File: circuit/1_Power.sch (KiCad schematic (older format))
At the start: 4 parts

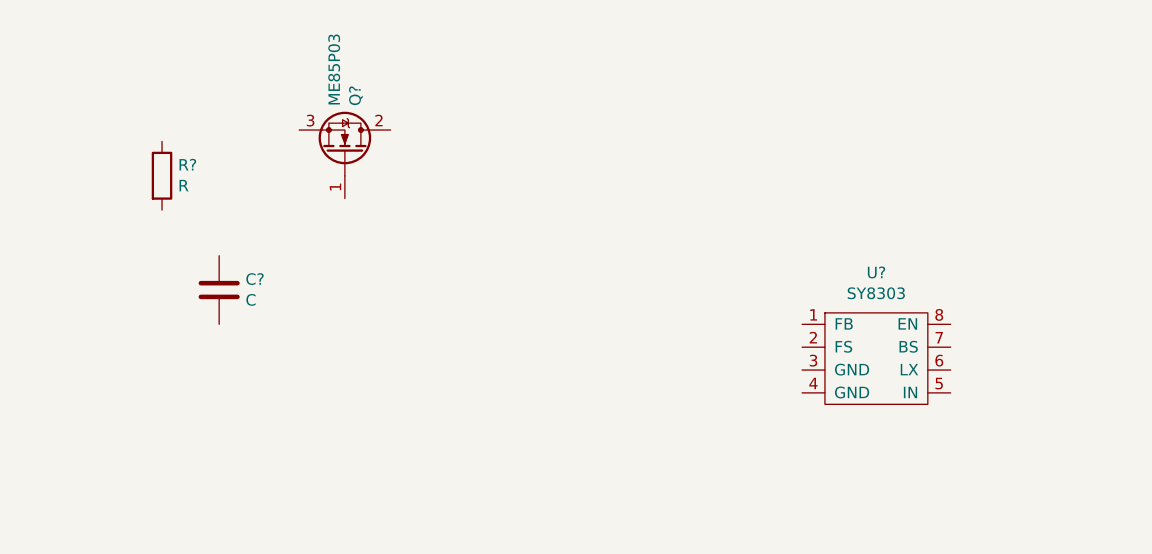
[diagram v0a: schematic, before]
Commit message: Power on delay and key switch circuit are added
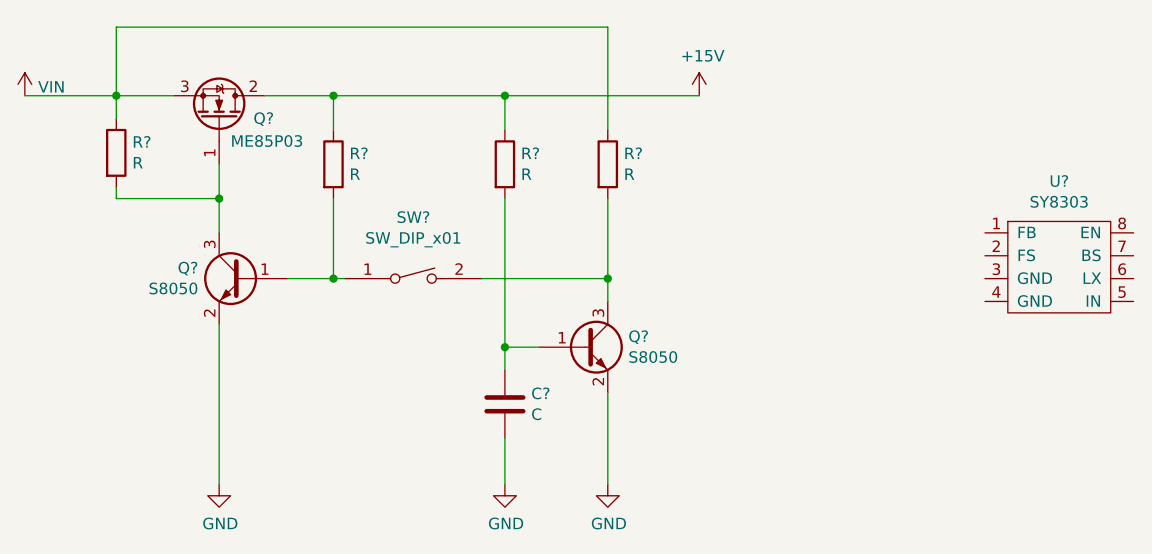
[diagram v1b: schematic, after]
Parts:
- added PWR?: VIN, symbol power:VIN
- added Q? (x2): S8050, Package_TO_SOT_SMD:SOT-23, symbol MM32_Periph:S8050
- added R? (x3): R, symbol Device:R
- added SW?: SW_DIP_x01, symbol Switch:SW_DIP_x01
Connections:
- net +15V: now reaches R?.1
- net +15V: now also Q?.2 (D), R?.1
- net at R?.2: now also C?.1, Q?.1 (B)
- net GND: now reaches C?.2
- net GND: now also Q?.2 (E), Q?.2 (E)
- net at Q?.1 (G): now also Q?.3 (C), R?.2
- net VDD: now reaches Q?.3 (S)
- net VDD: now also PWR?.1 (VDD), R?.1, R?.1
- new net: Q?.3 (C), R?.2, SW?.2
- new net: Q?.1 (B), R?.2, SW?.1
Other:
- moved on the sheet: C?, Q?, R?, U?
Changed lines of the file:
@@
 L MM32_Periph:SY8303 U?
 U 1 1 6191870D
-P 5150 3150
-F 0 "U?" H 5375 3725 50  0000 C CNN
-F 1 "SY8303" H 5375 3634 50  0000 C CNN
-F 2 "Package_TO_SOT_SMD:SOT-23-8" H 5800 3000 50  0001 C CNN
-F 3 "" H 5150 3300 50  0001 C CNN
-	1    5150 3150
+P 5950 2750
+F 0 "U?" H 6175 3325 50  0000 C CNN
+F 1 "SY8303" H 6175 3234 50  0000 C CNN
+F 2 "Package_TO_SOT_SMD:SOT-23-8" H 6600 2600 50  0001 C CNN
+F 3 "" H 5950 2900 50  0001 C CNN
+	1    5950 2750
 	1    0    0    -1
 $EndComp
@@
 L MM32_Periph:ME85P03 Q?
 U 1 1 61918BD3
-P 2850 2250
-F 0 "Q?" H 3255 2496 50  0000 L CNN
-F 1 "ME85P03" H 3255 2405 50  0000 L CNN
-F 2 "Package_TO_SOT_SMD:TO-252-2" H 3200 1950 50  0001 C CNN
-F 3 "" H 3300 2400 50  0001 C CNN
-	1    2850 2250
+P 2300 2100
+F 0 "Q?" V 2500 2450 50  0000 L CNN
+F 1 "ME85P03" V 2400 2350 50  0000 L CNN
+F 2 "Package_TO_SOT_SMD:TO-252-2" H 2650 1800 50  0001 C CNN
+F 3 "" H 2750 2250 50  0001 C CNN
+	1    2300 2100
 	0    1    -1   0
 $EndComp
@@
 L Device:R R?
 U 1 1 6190F774
-P 2250 2150
-F 0 "R?" H 2320 2196 50  0000 L CNN
-F 1 "R" H 2320 2105 50  0000 L CNN
-F 2 "" V 2180 2150 50  0001 C CNN
-F 3 "~" H 2250 2150 50  0001 C CNN
-	1    2250 2150
+P 3750 2100
+F 0 "R?" H 3820 2146 50  0000 L CNN
+F 1 "R" H 3820 2055 50  0000 L CNN
+F 2 "" V 3680 2100 50  0001 C CNN
+F 3 "~" H 3750 2100 50  0001 C CNN
+	1    3750 2100
 	1    0    0    -1
 $EndComp
@@
 L Device:C C?
 U 1 1 6190FF38
-P 2500 2650
-F 0 "C?" H 2615 2696 50  0000 L CNN
-F 1 "C" H 2615 2605 50  0000 L CNN
-F 2 "" H 2538 2500 50  0001 C CNN
-F 3 "~" H 2500 2650 50  0001 C CNN
-	1    2500 2650
-	1    0    0    -1
-$EndComp
+P 3750 3150
+F 0 "C?" H 3865 3196 50  0000 L CNN
+F 1 "C" H 3865 3105 50  0000 L CNN
+F 2 "" H 3788 3000 50  0001 C CNN
+F 3 "~" H 3750 3150 50  0001 C CNN
+	1    3750 3150
+	1    0    0    -1
+$EndComp
+$Comp
+L MM32_Periph:S8050 Q?
+U 1 1 61925CBB
+P 3900 3100
+F 0 "Q?" H 4290 3346 50  0000 L CNN
+F 1 "S8050" H 4290 3255 50  0000 L CNN
+F 2 "Package_TO_SOT_SMD:SOT-23" H 4850 3150 50  0001 C CNN
+F 3 "" H 4300 3350 50  0001 C CNN
+	1    3900 3100
+	1    0    0    -1
+$EndComp
+$Comp
+L Device:R R?
+U 1 1 6192BF14
+P 4200 2100
+F 0 "R?" H 4270 2146 50  0000 L CNN
+F 1 "R" H 4270 2055 50  0000 L CNN
+F 2 "" V 4130 2100 50  0001 C CNN
+F 3 "~" H 4200 2100 50  0001 C CNN
+	1    4200 2100
+	1    0    0    -1
+$EndComp
+Wire Wire Line
+	3900 2900 3750 2900
+Connection ~ 3750 2900
+Wire Wire Line
+	3750 2900 3750 3000
+$Comp
+L MM32_Periph:S8050 Q?
+U 1 1 6192C855
+P 2800 2800
+F 0 "Q?" H 3191 3046 50  0000 L CNN
+F 1 "S8050" H 3191 2955 50  0000 L CNN
+F 2 "Package_TO_SOT_SMD:SOT-23" H 3750 2850 50  0001 C CNN
+F 3 "" H 3200 3050 50  0001 C CNN
+	1    2800 2800
+	-1   0    0    -1
+$EndComp
+$Comp
+L Device:R R?
+U 1 1 6192FE42
+P 2050 2050
+F 0 "R?" H 2120 2096 50  0000 L CNN
+F 1 "R" H 2120 2005 50  0000 L CNN
+F 2 "" V 1980 2050 50  0001 C CNN
+F 3 "~" H 2050 2050 50  0001 C CNN
+	1    2050 2050
+	1    0    0    -1
+$EndComp
+Wire Wire Line
+	2050 2200 2050 2250
+Wire Wire Line
+	2050 2250 2500 2250
+Wire Wire Line
+	2500 2250 2500 2100
+Connection ~ 2500 2250
+Wire Wire Line
+	2300 1800 2050 1800
+Wire Wire Line
+	2050 1800 2050 1900
+Wire Wire Line
+	3750 2250 3750 2900
+Wire Wire Line
+	4200 2250 4200 2600
+Wire Wire Line
+	2050 1500 2050 1800
+Connection ~ 2050 1800
+$Comp
+L Device:R R?
+U 1 1 619359DE
+P 3000 2100
+F 0 "R?" H 3070 2146 50  0000 L CNN
+F 1 "R" H 3070 2055 50  0000 L CNN
+F 2 "" V 2930 2100 50  0001 C CNN
+F 3 "~" H 3000 2100 50  0001 C CNN
+	1    3000 2100
+	1    0    0    -1
+$EndComp
+Wire Wire Line
+	3750 1800 3750 1950
+Wire Wire Line
+	2700 1800 3000 1800
+Wire Wire Line
+	4200 1500 4200 1950
+Wire Wire Line
+	2050 1500 4200 1500
+Wire Wire Line
+	2500 2250 2500 2400
+$Comp
+L Switch:SW_DIP_x01 SW?
+U 1 1 6193A021
+P 3350 2600
+F 0 "SW?" H 3350 2867 50  0000 C CNN
+F 1 "SW_DIP_x01" H 3350 2776 50  0000 C CNN
+F 2 "" H 3350 2600 50  0001 C CNN
+F 3 "~" H 3350 2600 50  0001 C CNN
+	1    3350 2600
+	1    0    0    -1
+$EndComp
+Wire Wire Line
+	3000 1950 3000 1800
+Connection ~ 3000 1800
+Wire Wire Line
+	3000 1800 3750 1800
+Wire Wire Line
+	2800 2600 3000 2600
+Wire Wire Line
+	3000 2250 3000 2600
+Connection ~ 3000 2600
+Wire Wire Line
+	3000 2600 3050 2600
+Wire Wire Line
+	3650 2600 4200 2600
+Connection ~ 4200 2600
+Wire Wire Line
+	4200 2600 4200 2700
+$Comp
+L power:GND #PWR?
+U 1 1 6193E6CC
+P 3750 3500
+F 0 "#PWR?" H 3750 3250 50  0001 C CNN
+F 1 "GND" H 3755 3327 50  0000 C CNN
+F 2 "" H 3750 3500 50  0001 C CNN
+F 3 "" H 3750 3500 50  0001 C CNN
+	1    3750 3500
+	1    0    0    -1
+$EndComp
+$Comp
+L power:GND #PWR?
+U 1 1 6193E8C3
+P 4200 3500
+F 0 "#PWR?" H 4200 3250 50  0001 C CNN
+F 1 "GND" H 4205 3327 50  0000 C CNN
+F 2 "" H 4200 3500 50  0001 C CNN
+F 3 "" H 4200 3500 50  0001 C CNN
+	1    4200 3500
+	1    0    0    -1
+$EndComp
+$Comp
+L power:GND #PWR?
+U 1 1 6193EB71
+P 2500 3500
+F 0 "#PWR?" H 2500 3250 50  0001 C CNN
+F 1 "GND" H 2505 3327 50  0000 C CNN
+F 2 "" H 2500 3500 50  0001 C CNN
+F 3 "" H 2500 3500 50  0001 C CNN
+	1    2500 3500
+	1    0    0    -1
+$EndComp
+Wire Wire Line
+	2500 2800 2500 3500
+Wire Wire Line
+	3750 3300 3750 3500
+Wire Wire Line
+	4200 3100 4200 3500
+Wire Wire Line
+	3750 1800 4600 1800
+Connection ~ 3750 1800
+$Comp
+L power:VIN PWR?
+U 1 1 61943E9A
+P 1650 1800
+F 0 "PWR?" H 1650 1700 50  0001 C CNN
+F 1 "VIN" H 1708 1837 50  0000 L CNN
+F 2 "" H 1650 1800 50  0001 C CNN
+F 3 "" H 1650 1800 50  0001 C CNN
+	1    1650 1800
+	1    0    0    -1
+$EndComp
+$Comp
+L power:+15V #PWR?
+U 1 1 61945791
+P 4600 1800
+F 0 "#PWR?" H 4600 1650 50  0001 C CNN
+F 1 "+15V" H 4615 1973 50  0000 C CNN
+F 2 "" H 4600 1800 50  0001 C CNN
+F 3 "" H 4600 1800 50  0001 C CNN
+	1    4600 1800
+	1    0    0    -1
+$EndComp
+Wire Wire Line
+	1650 1800 2050 1800
 $EndSCHEMATC
